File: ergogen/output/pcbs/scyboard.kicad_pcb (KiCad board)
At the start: 2 copper layers, 143.9 x 96.5 mm, 54 parts

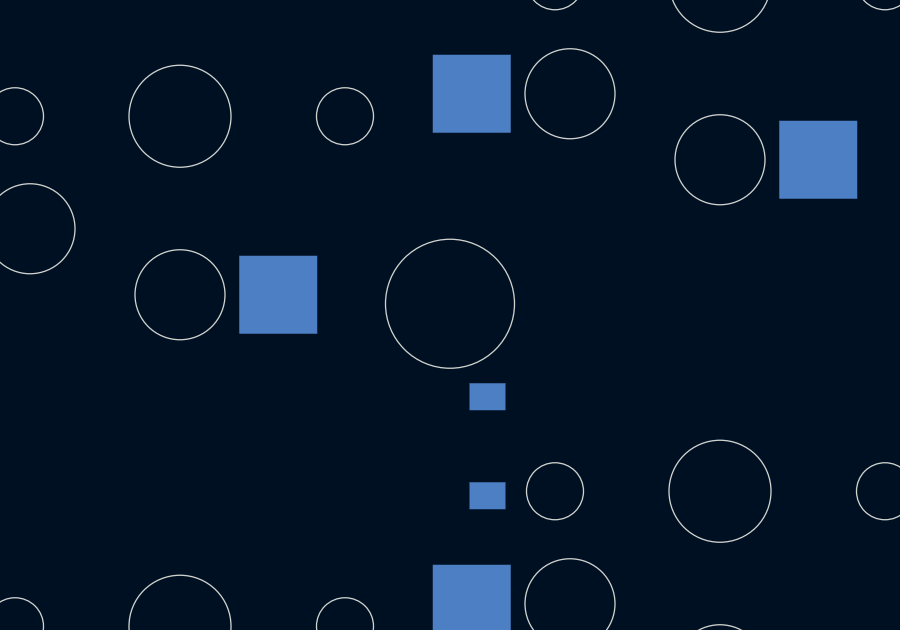
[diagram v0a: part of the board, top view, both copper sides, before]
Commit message: Compile
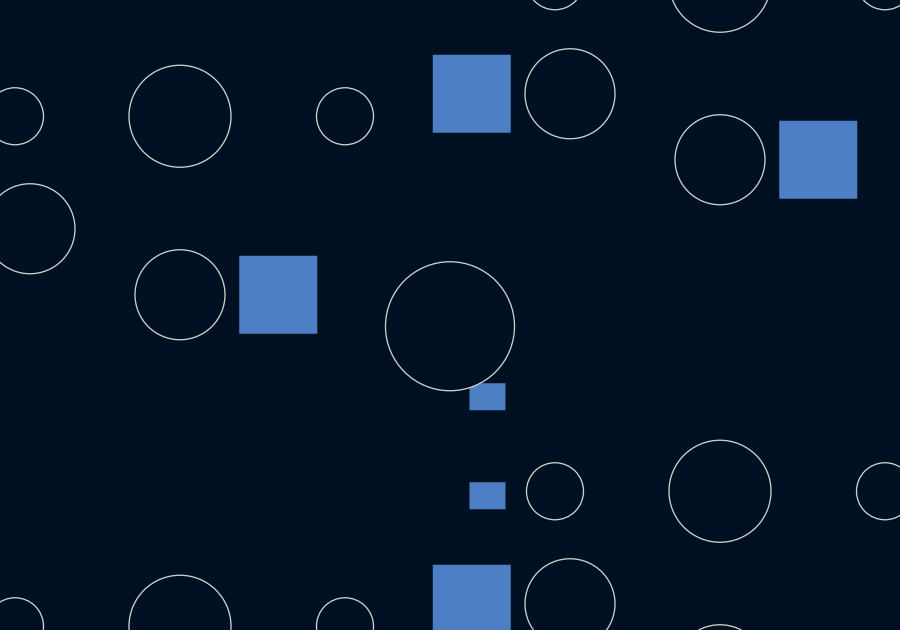
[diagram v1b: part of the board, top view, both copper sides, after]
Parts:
- moved MH4 0.75 mm to (95.0, 59.3)
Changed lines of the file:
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@@
   (footprint "ceoloide:mounting_hole_npth"
     (layer "F.Cu")
-    (at 95 58.56999999999999 0)
+    (at 95 59.31999999999999 0)
     (property "Reference" "MH4"
       (at 0 2.55 0)

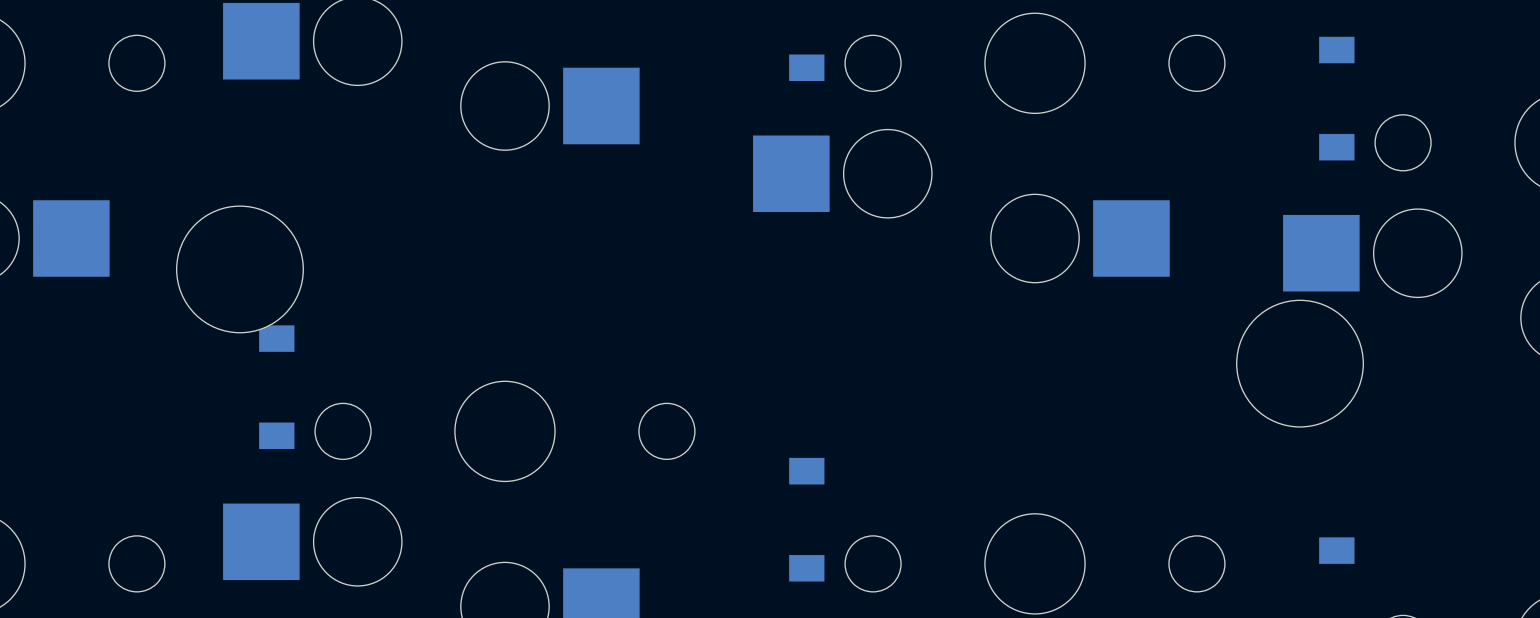
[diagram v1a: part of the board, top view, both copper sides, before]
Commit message: Compile
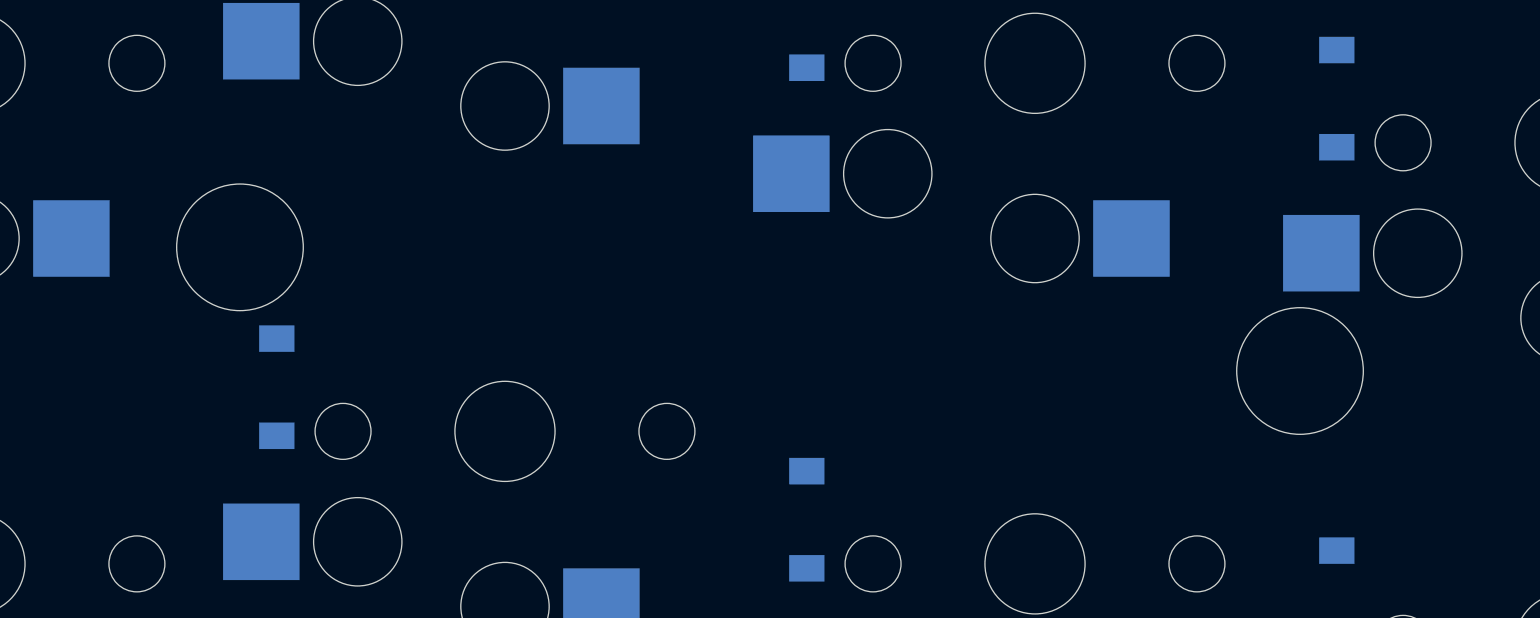
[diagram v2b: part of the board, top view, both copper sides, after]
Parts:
- moved MH4 0.75 mm to (95.0, 58.6)
- moved MH5 0.25 mm to (131.0, 62.8)
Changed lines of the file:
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@@
   (footprint "ceoloide:mounting_hole_npth"
     (layer "F.Cu")
-    (at 95 59.31999999999999 0)
+    (at 95 58.56999999999999 0)
     (property "Reference" "MH4"
       (at 0 2.55 0)
@@
   (footprint "ceoloide:mounting_hole_npth"
     (layer "F.Cu")
-    (at 131 62.519999999999996 0)
+    (at 131 62.769999999999996 0)
     (property "Reference" "MH5"
       (at 0 2.55 0)

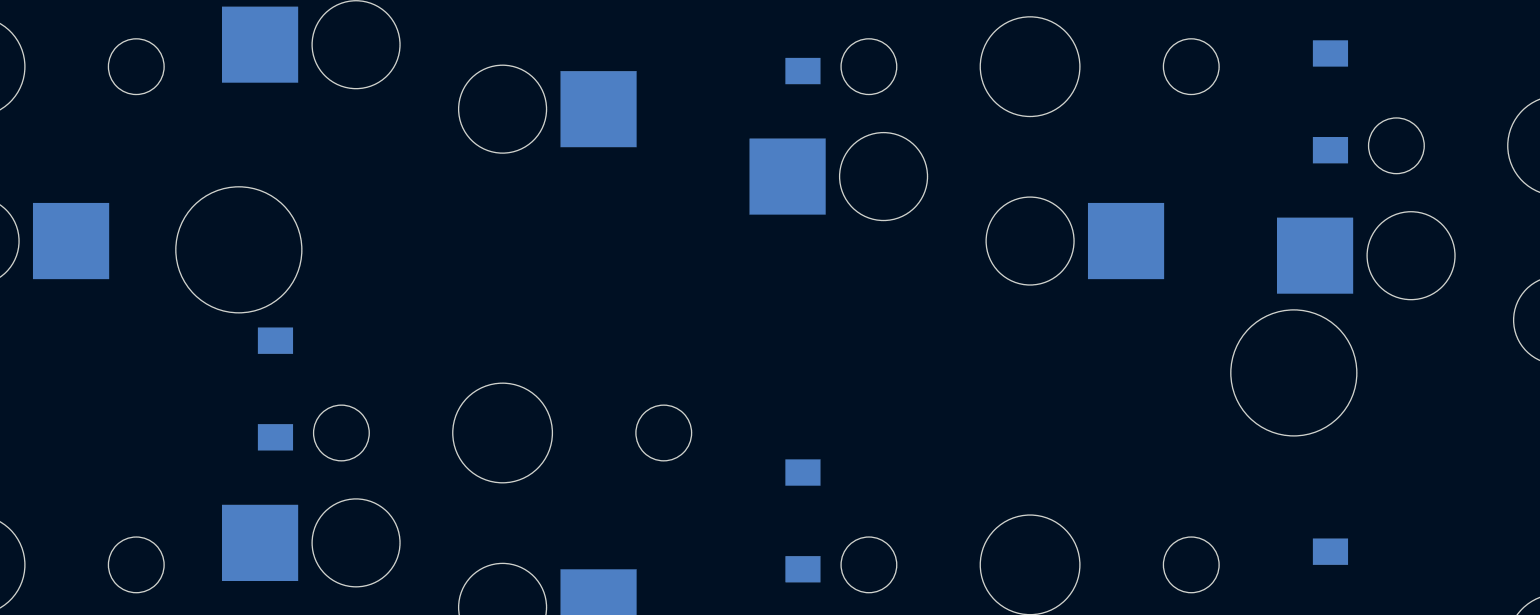
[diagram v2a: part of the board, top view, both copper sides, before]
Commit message: Compile
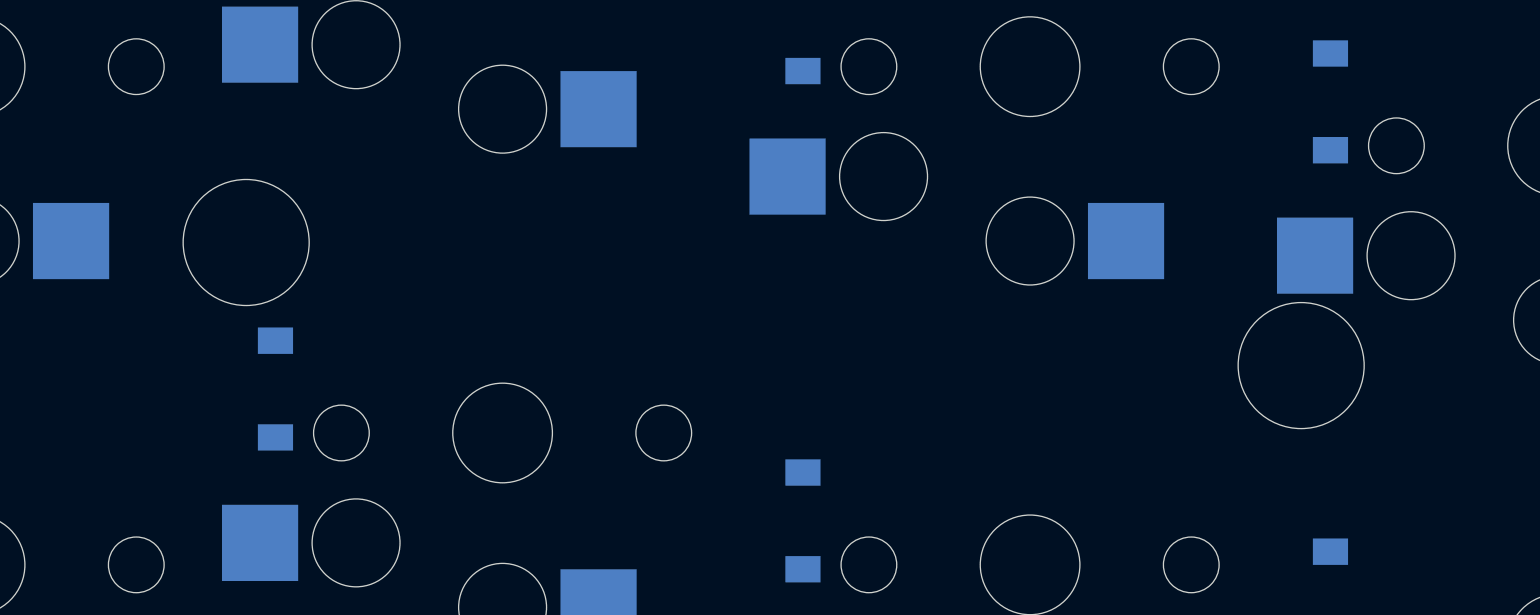
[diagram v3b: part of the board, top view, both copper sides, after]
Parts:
- moved MH4 0.35 mm to (95.2, 58.3)
- moved MH5 0.35 mm to (131.2, 62.5)
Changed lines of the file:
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@@
   (footprint "ceoloide:mounting_hole_npth"
     (layer "F.Cu")
-    (at 95 58.56999999999999 0)
+    (at 95.25 58.31999999999999 0)
     (property "Reference" "MH4"
       (at 0 2.55 0)
@@
   (footprint "ceoloide:mounting_hole_npth"
     (layer "F.Cu")
-    (at 131 62.769999999999996 0)
+    (at 131.25 62.519999999999996 0)
     (property "Reference" "MH5"
       (at 0 2.55 0)

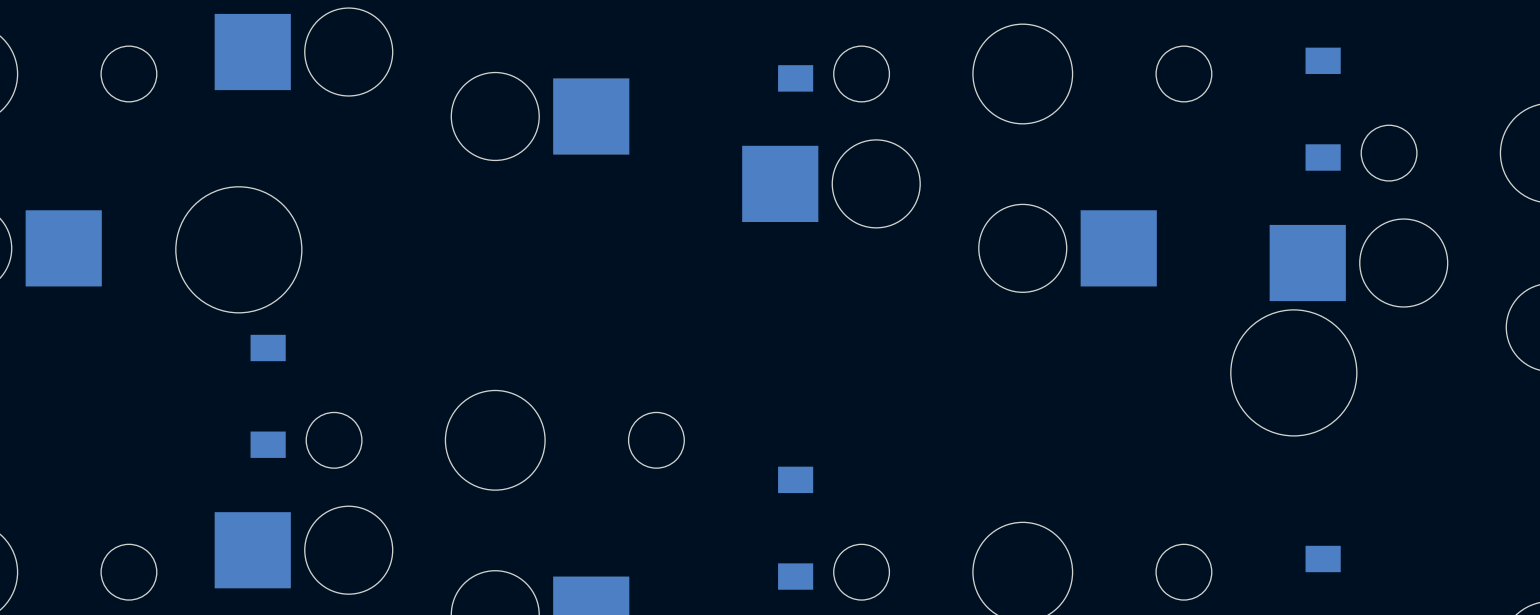
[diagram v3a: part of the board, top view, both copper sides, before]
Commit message: Compile
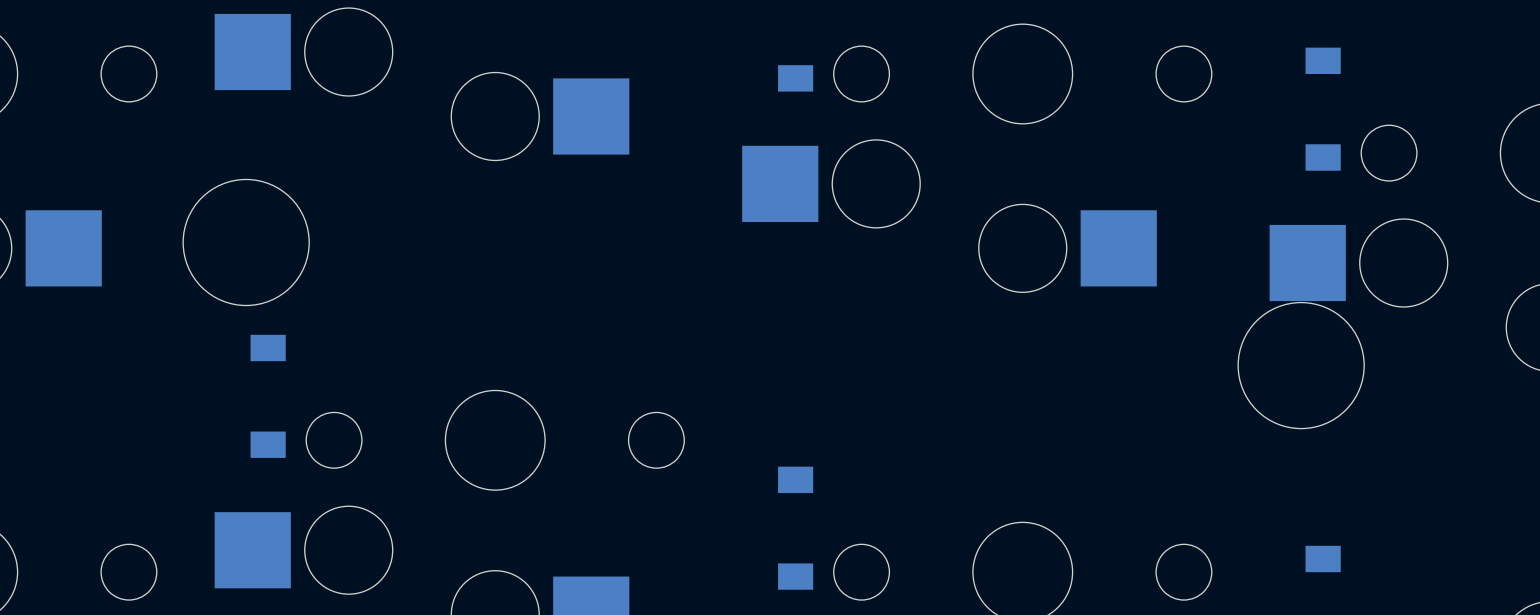
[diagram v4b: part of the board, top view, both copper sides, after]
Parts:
- moved MH4 0.35 mm to (95.5, 58.1)
- moved MH5 0.35 mm to (131.5, 62.3)
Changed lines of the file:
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@@
   (footprint "ceoloide:mounting_hole_npth"
     (layer "F.Cu")
-    (at 95.25 58.31999999999999 0)
+    (at 95.5 58.06999999999999 0)
     (property "Reference" "MH4"
       (at 0 2.55 0)
@@
   (footprint "ceoloide:mounting_hole_npth"
     (layer "F.Cu")
-    (at 131.25 62.519999999999996 0)
+    (at 131.5 62.269999999999996 0)
     (property "Reference" "MH5"
       (at 0 2.55 0)

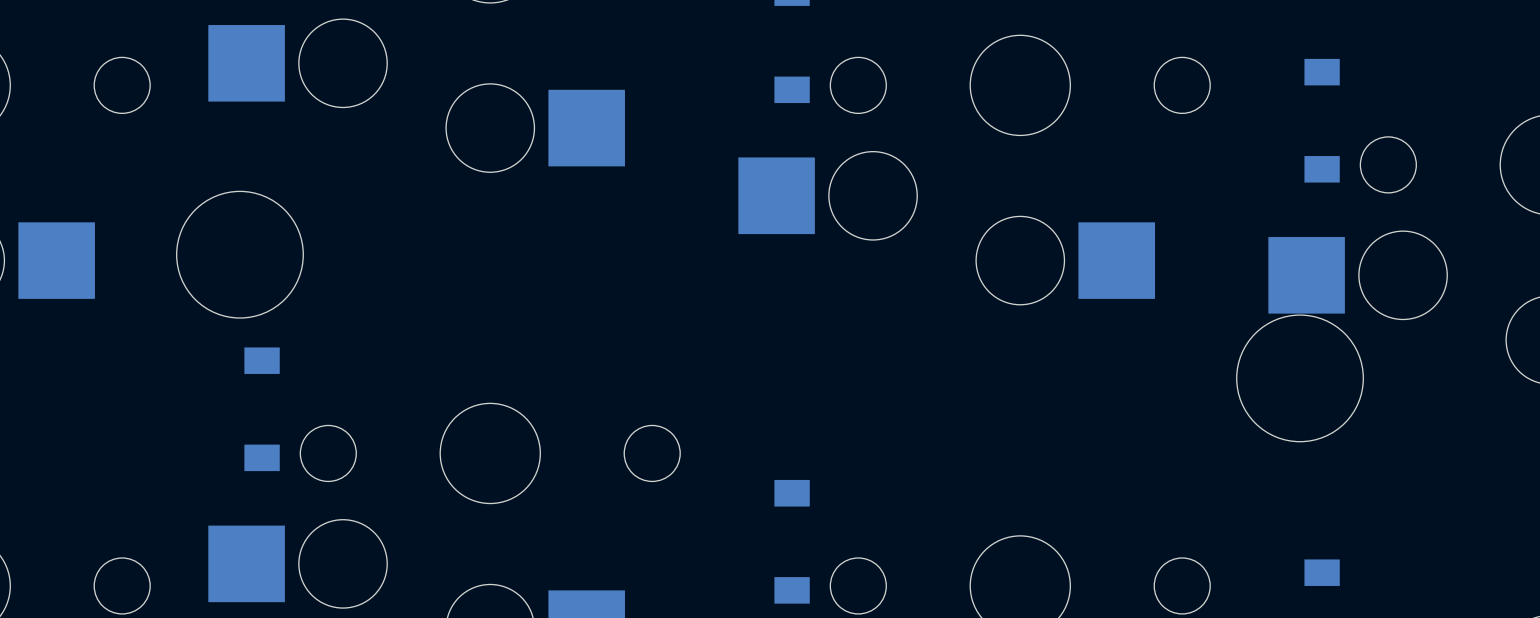
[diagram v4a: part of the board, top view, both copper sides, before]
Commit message: Compile
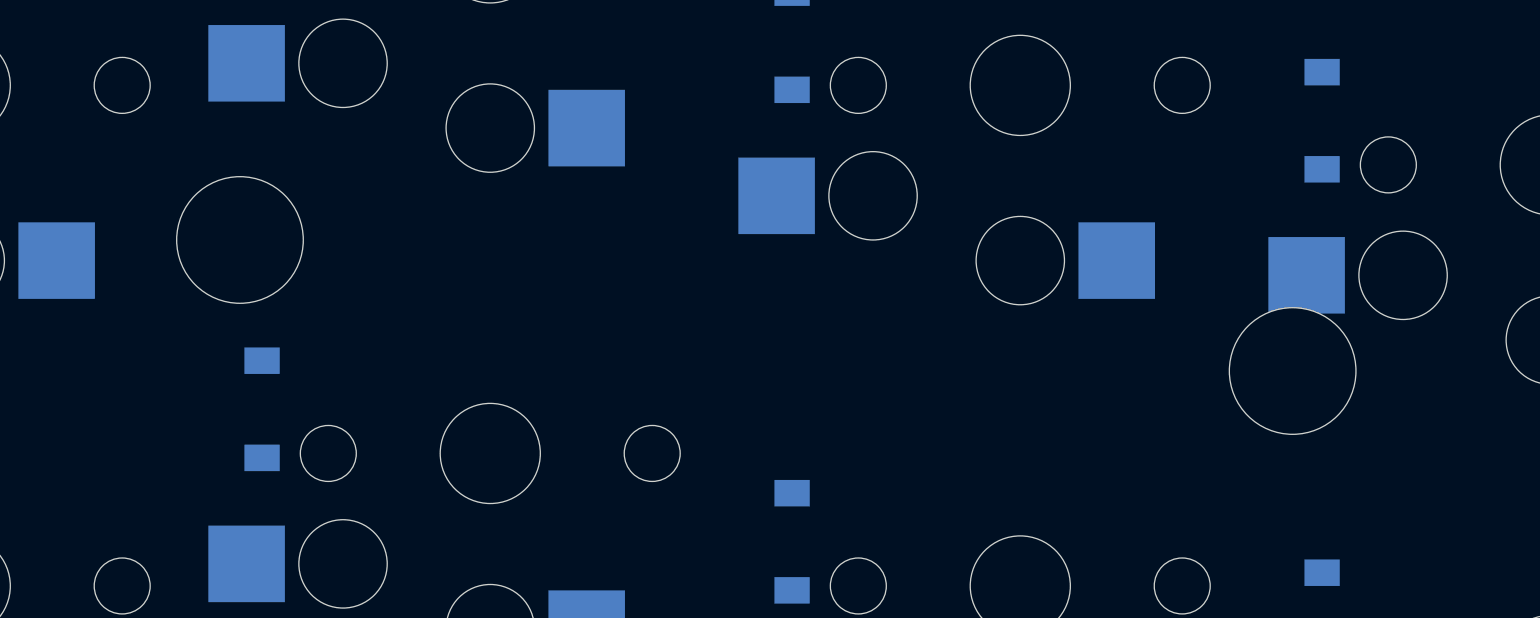
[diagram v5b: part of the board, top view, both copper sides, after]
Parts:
- moved MH4 0.50 mm to (95.5, 57.6)
- moved MH5 0.35 mm to (131.2, 62.0)
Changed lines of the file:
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@@
   (footprint "ceoloide:mounting_hole_npth"
     (layer "F.Cu")
-    (at 95.5 58.06999999999999 0)
+    (at 95.5 57.56999999999999 0)
     (property "Reference" "MH4"
       (at 0 2.55 0)
@@
   (footprint "ceoloide:mounting_hole_npth"
     (layer "F.Cu")
-    (at 131.5 62.269999999999996 0)
+    (at 131.25 62.019999999999996 0)
     (property "Reference" "MH5"
       (at 0 2.55 0)
